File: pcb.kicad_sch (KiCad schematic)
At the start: 13 parts, among them J1 vik-module-connector, J2 Conn_01x12_Pin, J3 vik-module-connector, Q1 S8050

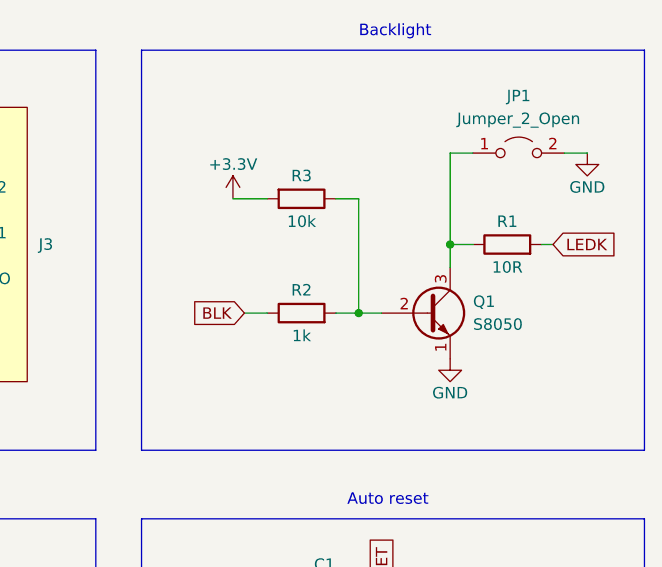
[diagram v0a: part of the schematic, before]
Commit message: v0.2
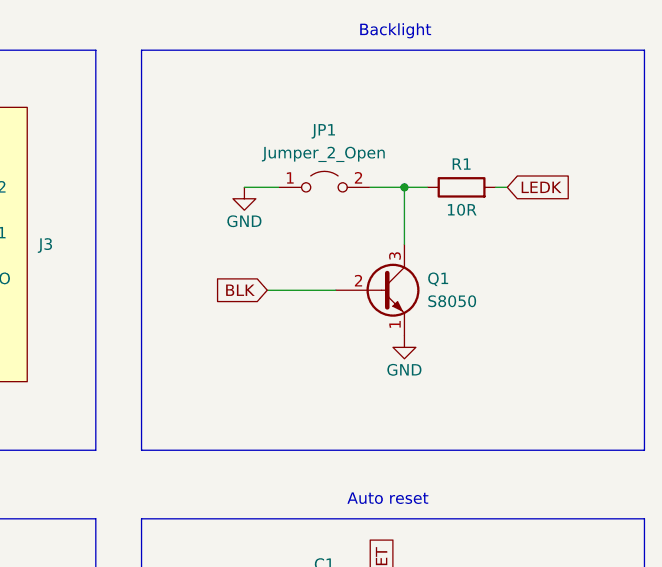
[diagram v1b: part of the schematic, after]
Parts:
- removed R2: 1k, Resistor_SMD:R_1206_3216Metric_Pad1.30x1.75mm_HandSolder, symbol Device:R
- removed R3: 10k, Resistor_SMD:R_1206_3216Metric_Pad1.30x1.75mm_HandSolder, symbol Device:R
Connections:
- net BLK: now also Q1.2 (B)
- net GND: now also JP1.1 (A); no longer JP1.2 (B)
- net at Q1.3 (C), R1.1: now also JP1.2 (B); no longer JP1.1 (A)
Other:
- moved on the sheet: Q1, R1
